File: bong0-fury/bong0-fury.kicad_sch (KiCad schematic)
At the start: 0 parts

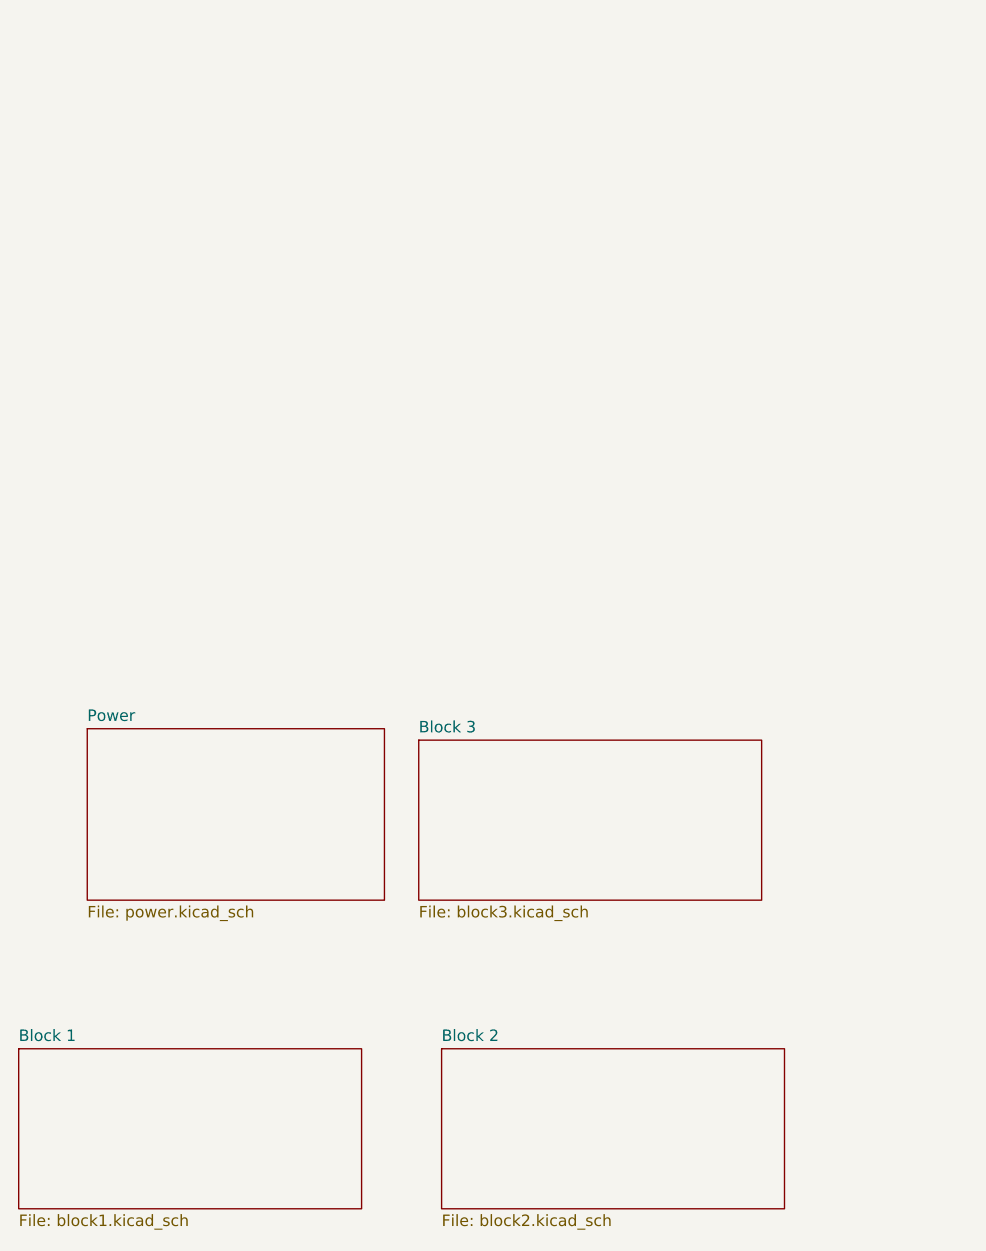
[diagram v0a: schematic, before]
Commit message: Unknown changes
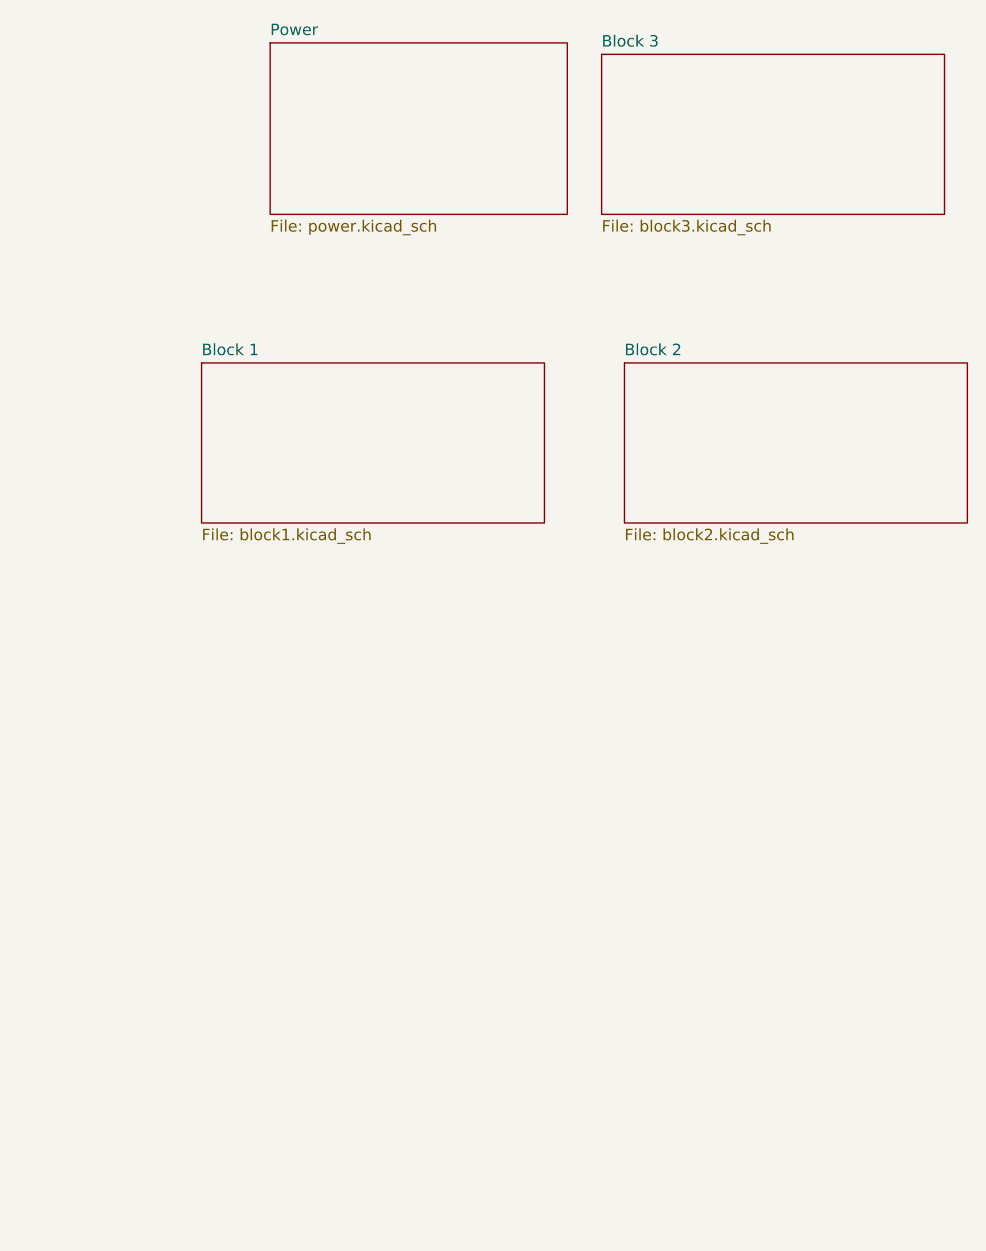
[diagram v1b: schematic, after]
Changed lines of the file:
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@@
 	)
 	(sheet
-		(at 93.98 144.78)
+		(at 114.3 68.58)
 		(size 38.1 17.78)
 		(fields_autoplaced yes)
@@
 		)
 		(property "Sheetname" "Block 3"
-			(at 93.98 144.0684 0)
+			(at 114.3 67.8684 0)
 			(effects
 				(font
@@
 		)
 		(property "Sheetfile" "block3.kicad_sch"
-			(at 93.98 163.1446 0)
+			(at 114.3 86.9446 0)
 			(effects
 				(font
@@
 	)
 	(sheet
-		(at 57.15 143.51)
+		(at 77.47 67.31)
 		(size 33.02 19.05)
 		(fields_autoplaced yes)
@@
 		)
 		(property "Sheetname" "Power"
-			(at 57.15 142.7984 0)
+			(at 77.47 66.5984 0)
 			(effects
 				(font
@@
 		)
 		(property "Sheetfile" "power.kicad_sch"
-			(at 57.15 163.1446 0)
+			(at 77.47 86.9446 0)
 			(effects
 				(font
@@
 	)
 	(sheet
-		(at 96.52 179.07)
+		(at 116.84 102.87)
 		(size 38.1 17.78)
 		(fields_autoplaced yes)
@@
 		)
 		(property "Sheetname" "Block 2"
-			(at 96.52 178.3584 0)
+			(at 116.84 102.1584 0)
 			(effects
 				(font
@@
 		)
 		(property "Sheetfile" "block2.kicad_sch"
-			(at 96.52 197.4346 0)
+			(at 116.84 121.2346 0)
 			(effects
 				(font
@@
 	)
 	(sheet
-		(at 49.53 179.07)
+		(at 69.85 102.87)
 		(size 38.1 17.78)
 		(fields_autoplaced yes)
@@
 		)
 		(property "Sheetname" "Block 1"
-			(at 49.53 178.3584 0)
+			(at 69.85 102.1584 0)
 			(effects
 				(font
@@
 		)
 		(property "Sheetfile" "block1.kicad_sch"
-			(at 49.53 197.4346 0)
+			(at 69.85 121.2346 0)
 			(effects
 				(font
